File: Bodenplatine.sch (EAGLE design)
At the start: 113 parts, among them K1 RY612012, K2 RY612012, K3 RY612012, K4 RY612012, K5 RY612012, K6 RY612012, K7 RY612012, K8 RY612012, K9 RY612012, Q1 BC846BLT1SMD, Q2 BC846BLT1SMD, Q3 BC846BLT1SMD, Q4 BC846BLT1SMD, Q5 BC846BLT1SMD, Q6 BC846BLT1SMD, Q7 BC846BLT1SMD, Q8 BC846BLT1SMD, Q9 BC846BLT1SMD, X1 SPRINGCON_AST125_5X2, X10 SPRINGCON_AST125_3X2, X11 SPRINGCON_AST125_4X2, X12 SPRINGCON_AST125_4X2, X13 SPRINGCON_AST125_5X2, X14 236-403, X15 236-402, X2 SPRINGCON_AST125_5X2, X3 SPRINGCON_AST125_5X2, X4 SPRINGCON_AST125_5X2, X5 SPRINGCON_AST125_5X2, X6 SPRINGCON_AST125_5X2, X7 SPRINGCON_AST125_5X2, X8 SPRINGCON_AST125_5X2, X9 SPRINGCON_AST125_5X2

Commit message: Erste Version der 1.0.0 Produktionsdaten
Versuch alle Datenblätter, eine Kalkulation und Lagerverwaltung und
einer Eagle Datei mit "nur SMD" Bestückungsvariante. Zur Zeit noch nicht
fertig.
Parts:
- F1, F10, F12, F13, F2, F3, F4, F5, F6, F7, F8, F9: MF (none) -> SCHURTER; MPN (none) -> 3101.0040; OC_FARNELL unknown -> 1222690
- JP1: device xMZ-Mod-Touch-Bodenplatine:PINHD-2X10 -> Bodenplatine:PINHD-2X10; MF TE CONNECTIVITY / AMP -> (none); MPN 825440-5 -> (none); OC_CONRAD (none) -> 739630 - 62; OC_FARNELL 3417773 -> unknown
- Q1, Q2, Q3, Q4, Q5, Q6, Q7, Q8, Q9: MF ON SEMICONDUCTOR -> NXP; MPN BC846BWT1G -> BC846,215; OC_FARNELL 2317836 -> 1081227
- V1, V10, V11, V12, V17, V2, V3, V4, V9: OC_FARNELL (none) -> 2453275
- X1, X13, X2, X3, X4, X5, X6, X7, X8, X9: OC_METZ-CONNECT (none) -> AST12510
- X10: OC_METZ-CONNECT (none) -> AST1256
- X11: OC_METZ-CONNECT (none) -> AST1258

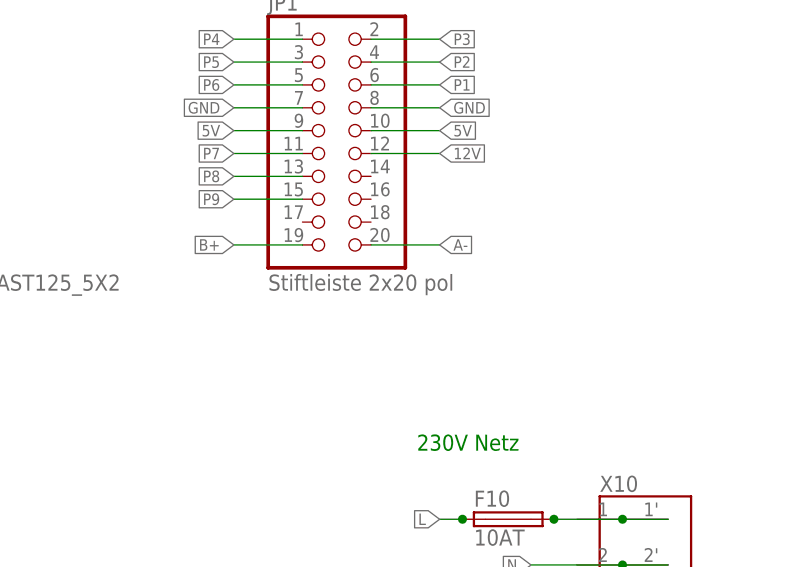
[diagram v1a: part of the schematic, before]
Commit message: Produktionsdaten exportiert. v1.0.0 soweit fertig
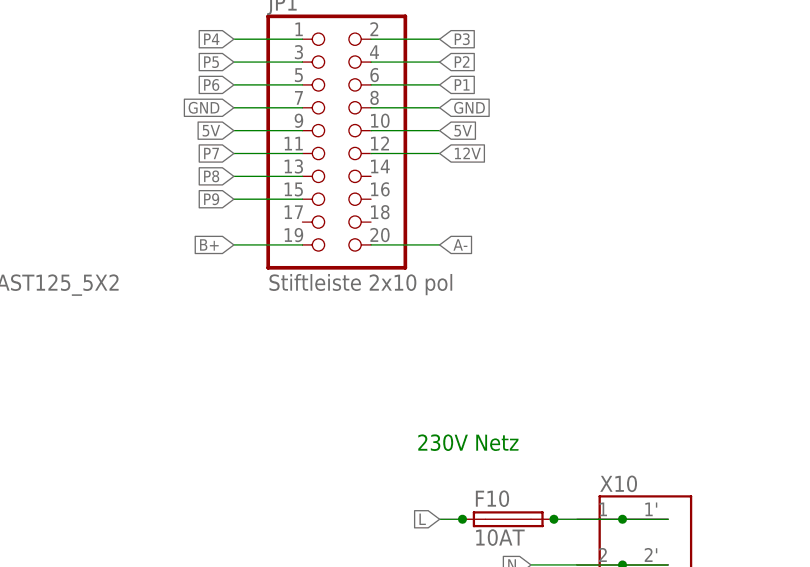
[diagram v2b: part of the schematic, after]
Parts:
- JP1: value Stiftleiste 2x20 pol -> Stiftleiste 2x10 pol; device Bodenplatine:PINHD-2X10 -> xMZ-Mod-Touch-Bodenplatine:PINHD-2X10
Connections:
- net 12V: no longer F12.1@2, F13.1@2
- net L: no longer F10.1@2
- net N$1: no longer F2.1@2
- net N$12: no longer F3.2@2
- net N$19: no longer F3.1@2
- net N$22: no longer F4.2@2
- net N$29: no longer F4.1@2
- net N$3: no longer F2.2@2
- net N$32: no longer F5.2@2
- net N$39: no longer F5.1@2
- net N$42: no longer F6.2@2
- net N$49: no longer F6.1@2
- net N$52: no longer F7.2@2
- net N$59: no longer F7.1@2
- net N$62: no longer F8.2@2
- net N$69: no longer F8.1@2
- net N$72: no longer F9.2@2
- net N$79: no longer F9.1@2
- net N$82: no longer F1.2@2
- net N$89: no longer F1.1@2
- net N$91: no longer F10.2@2
- net N$92: no longer F13.2@2
- net N$94: no longer F12.2@2
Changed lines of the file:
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@@
 </attributes>
 <variantdefs>
-<variantdef name="nur SMD"/>
+<variantdef name="nur SMD" current="yes"/>
 </variantdefs>
 <classes>
@@
 <variant name="nur SMD" populate="no"/>
 </part>
-<part name="JP1" library="Bodenplatine" deviceset="PINHD-2X10" device="" value="Stiftleiste 2x20 pol">
+<part name="JP1" library="xMZ-Mod-Touch-Bodenplatine" deviceset="PINHD-2X10" device="" value="Stiftleiste 2x10 pol">
 <attribute name="MF" value=""/>
 <attribute name="MPN" value=""/>
@@
 <pinref part="F2" gate="G$1" pin="2"/>
 <wire x1="81.28" y1="180.34" x2="78.74" y2="180.34" width="0.1524" layer="91"/>
-<pinref part="F2" gate="G$1" pin="2@2"/>
+<pinref part="F2" gate="G$1" pin="2"/>
 <junction x="81.28" y="180.34"/>
 </segment>
@@
 <wire x1="101.6" y1="180.34" x2="106.68" y2="180.34" width="0.1524" layer="91"/>
 <junction x="101.6" y="180.34"/>
-<pinref part="F2" gate="G$1" pin="1@2"/>
+<pinref part="F2" gate="G$1" pin="1"/>
 <junction x="91.44" y="180.34"/>
 </segment>
@@
 <pinref part="F3" gate="G$1" pin="2"/>
 <wire x1="81.28" y1="129.54" x2="78.74" y2="129.54" width="0.1524" layer="91"/>
-<pinref part="F3" gate="G$1" pin="2@2"/>
+<pinref part="F3" gate="G$1" pin="2"/>
 <junction x="81.28" y="129.54"/>
 </segment>
@@
 <wire x1="99.06" y1="129.54" x2="104.14" y2="129.54" width="0.1524" layer="91"/>
 <junction x="99.06" y="129.54"/>
-<pinref part="F3" gate="G$1" pin="1@2"/>
+<pinref part="F3" gate="G$1" pin="1"/>
 <junction x="91.44" y="129.54"/>
 </segment>
@@
 <pinref part="F4" gate="G$1" pin="2"/>
 <wire x1="83.82" y1="78.74" x2="81.28" y2="78.74" width="0.1524" layer="91"/>
-<pinref part="F4" gate="G$1" pin="2@2"/>
+<pinref part="F4" gate="G$1" pin="2"/>
 <junction x="83.82" y="78.74"/>
 </segment>
@@
 <wire x1="101.6" y1="78.74" x2="106.68" y2="78.74" width="0.1524" layer="91"/>
 <junction x="101.6" y="78.74"/>
-<pinref part="F4" gate="G$1" pin="1@2"/>
+<pinref part="F4" gate="G$1" pin="1"/>
 <junction x="93.98" y="78.74"/>
 </segment>
@@
 <pinref part="F5" gate="G$1" pin="2"/>
 <wire x1="205.74" y1="233.68" x2="203.2" y2="233.68" width="0.1524" layer="91"/>
-<pinref part="F5" gate="G$1" pin="2@2"/>
+<pinref part="F5" gate="G$1" pin="2"/>
 <junction x="205.74" y="233.68"/>
 </segment>
@@
 <wire x1="223.52" y1="233.68" x2="228.6" y2="233.68" width="0.1524" layer="91"/>
 <junction x="223.52" y="233.68"/>
-<pinref part="F5" gate="G$1" pin="1@2"/>
+<pinref part="F5" gate="G$1" pin="1"/>
 <junction x="215.9" y="233.68"/>
 </segment>
@@
 <pinref part="F6" gate="G$1" pin="2"/>
 <wire x1="205.74" y1="180.34" x2="203.2" y2="180.34" width="0.1524" layer="91"/>
-<pinref part="F6" gate="G$1" pin="2@2"/>
+<pinref part="F6" gate="G$1" pin="2"/>
 <junction x="205.74" y="180.34"/>
 </segment>
@@
 <wire x1="223.52" y1="180.34" x2="228.6" y2="180.34" width="0.1524" layer="91"/>
 <junction x="223.52" y="180.34"/>
-<pinref part="F6" gate="G$1" pin="1@2"/>
+<pinref part="F6" gate="G$1" pin="1"/>
 <junction x="215.9" y="180.34"/>
 </segment>
@@
 <pinref part="F7" gate="G$1" pin="2"/>
 <wire x1="205.74" y1="129.54" x2="203.2" y2="129.54" width="0.1524" layer="91"/>
-<pinref part="F7" gate="G$1" pin="2@2"/>
+<pinref part="F7" gate="G$1" pin="2"/>
 <junction x="205.74" y="129.54"/>
 </segment>
@@
 <wire x1="223.52" y1="129.54" x2="228.6" y2="129.54" width="0.1524" layer="91"/>
 <junction x="223.52" y="129.54"/>
-<pinref part="F7" gate="G$1" pin="1@2"/>
+<pinref part="F7" gate="G$1" pin="1"/>
 <junction x="215.9" y="129.54"/>
 </segment>
@@
 <pinref part="F8" gate="G$1" pin="2"/>
 <wire x1="210.82" y1="78.74" x2="205.74" y2="78.74" width="0.1524" layer="91"/>
-<pinref part="F8" gate="G$1" pin="2@2"/>
+<pinref part="F8" gate="G$1" pin="2"/>
 <junction x="210.82" y="78.74"/>
 </segment>
@@
 <wire x1="226.06" y1="78.74" x2="231.14" y2="78.74" width="0.1524" layer="91"/>
 <junction x="226.06" y="78.74"/>
-<pinref part="F8" gate="G$1" pin="1@2"/>
+<pinref part="F8" gate="G$1" pin="1"/>
 <junction x="220.98" y="78.74"/>
 </segment>
@@
 <pinref part="F9" gate="G$1" pin="2"/>
 <wire x1="330.2" y1="233.68" x2="327.66" y2="233.68" width="0.1524" layer="91"/>
-<pinref part="F9" gate="G$1" pin="2@2"/>
+<pinref part="F9" gate="G$1" pin="2"/>
 <junction x="330.2" y="233.68"/>
 </segment>
@@
 <wire x1="347.98" y1="233.68" x2="353.06" y2="233.68" width="0.1524" layer="91"/>
 <junction x="347.98" y="233.68"/>
-<pinref part="F9" gate="G$1" pin="1@2"/>
+<pinref part="F9" gate="G$1" pin="1"/>
 <junction x="340.36" y="233.68"/>
 </segment>
@@
 <pinref part="F1" gate="G$1" pin="2"/>
 <wire x1="81.28" y1="233.68" x2="78.74" y2="233.68" width="0.1524" layer="91"/>
-<pinref part="F1" gate="G$1" pin="2@2"/>
+<pinref part="F1" gate="G$1" pin="2"/>
 <junction x="81.28" y="233.68"/>
 </segment>
@@
 <wire x1="99.06" y1="233.68" x2="104.14" y2="233.68" width="0.1524" layer="91"/>
 <junction x="99.06" y="233.68"/>
-<pinref part="F1" gate="G$1" pin="1@2"/>
+<pinref part="F1" gate="G$1" pin="1"/>
 <junction x="91.44" y="233.68"/>
 </segment>
@@
 <wire x1="327.66" y1="96.52" x2="325.12" y2="96.52" width="0.1524" layer="91"/>
 <label x="325.12" y="96.52" size="1.27" layer="95" rot="R180" xref="yes"/>
-<pinref part="F12" gate="G$1" pin="1@2"/>
+<pinref part="F12" gate="G$1" pin="1"/>
 <junction x="327.66" y="96.52"/>
 </segment>
@@
 <wire x1="330.2" y1="58.42" x2="327.66" y2="58.42" width="0.1524" layer="91"/>
 <label x="327.66" y="58.42" size="1.27" layer="95" rot="R180" xref="yes"/>
-<pinref part="F13" gate="G$1" pin="1@2"/>
+<pinref part="F13" gate="G$1" pin="1"/>
 <junction x="330.2" y="58.42"/>
 </segment>
@@
 <wire x1="287.02" y1="134.62" x2="284.48" y2="134.62" width="0.1524" layer="91"/>
 <label x="284.48" y="134.62" size="1.27" layer="95" rot="R180" xref="yes"/>
-<pinref part="F10" gate="G$1" pin="1@2"/>
+<pinref part="F10" gate="G$1" pin="1"/>
 <junction x="287.02" y="134.62"/>
 </segment>
@@
 <junction x="347.98" y="91.44"/>
 <junction x="347.98" y="96.52"/>
-<pinref part="F12" gate="G$1" pin="2@2"/>
+<pinref part="F12" gate="G$1" pin="2"/>
 <junction x="337.82" y="96.52"/>
 </segment>
@@
 <wire x1="353.06" y1="58.42" x2="347.98" y2="58.42" width="0.1524" layer="91"/>
 <junction x="347.98" y="58.42"/>
-<pinref part="F13" gate="G$1" pin="2@2"/>
+<pinref part="F13" gate="G$1" pin="2"/>
 <junction x="340.36" y="58.42"/>
 </segment>
@@
 <wire x1="309.88" y1="134.62" x2="304.8" y2="134.62" width="0.1524" layer="91"/>
 <pinref part="F10" gate="G$1" pin="2"/>
-<pinref part="F10" gate="G$1" pin="2@2"/>
+<pinref part="F10" gate="G$1" pin="2"/>
 <junction x="297.18" y="134.62"/>
 <pinref part="X10" gate="G$1" pin="1@1"/>
